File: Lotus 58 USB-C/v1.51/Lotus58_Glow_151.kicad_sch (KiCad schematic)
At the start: 151 parts, among them J1 HRO-TYPE-C-31-M-13x, P1 OLED, SW1 Kailh hotswap MX socket, SW10 Kailh hotswap MX socket, SW11 Kailh hotswap MX socket, SW12 Kailh hotswap MX socket, SW13 Kailh hotswap MX socket, SW14 Kailh hotswap MX socket, SW15 Kailh hotswap MX socket, SW16 Kailh hotswap MX socket, SW17 Kailh hotswap MX socket, SW18 Kailh hotswap MX socket, SW19 Kailh hotswap MX socket, SW2 Kailh hotswap MX socket, SW20 Kailh hotswap MX socket, SW21 Kailh hotswap MX socket, SW22 Kailh hotswap MX socket, SW23 Kailh hotswap MX socket, SW24 Kailh hotswap MX socket, SW25 Kailh hotswap MX socket, SW26 Kailh hotswap MX socket, SW27 Kailh hotswap MX socket, SW28 Kailh hotswap MX socket, SW29 Kailh hotswap MX socket, SW3 Kailh hotswap MX socket, SW4 Kailh hotswap MX socket, SW5 Kailh hotswap MX socket, SW6 Kailh hotswap MX socket, SW7 Kailh hotswap MX socket, SW8 Kailh hotswap MX socket, SW9 Kailh hotswap MX socket, U1 Controller, U2 SRV05-4, U3 SRV05-4

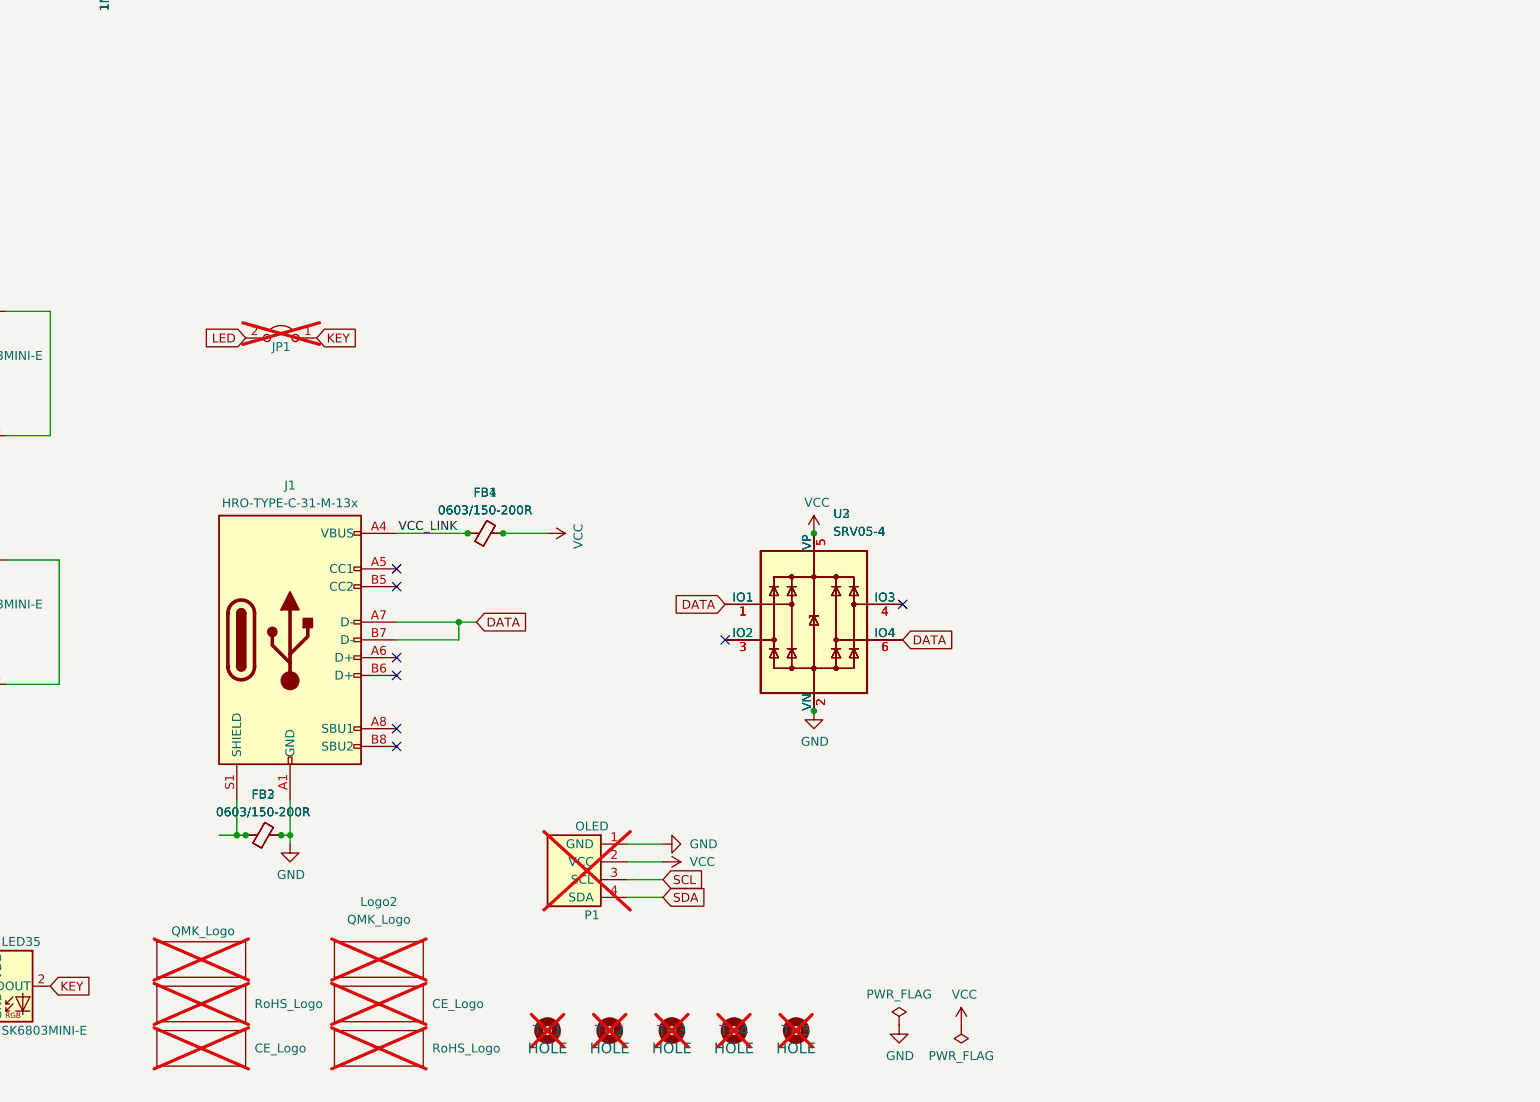
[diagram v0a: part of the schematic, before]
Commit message: Lotus 58 - TRRS Link v1.30
release ready

Signed-off-by: Markus Knutsson <markus.knutsson@tweety.se>
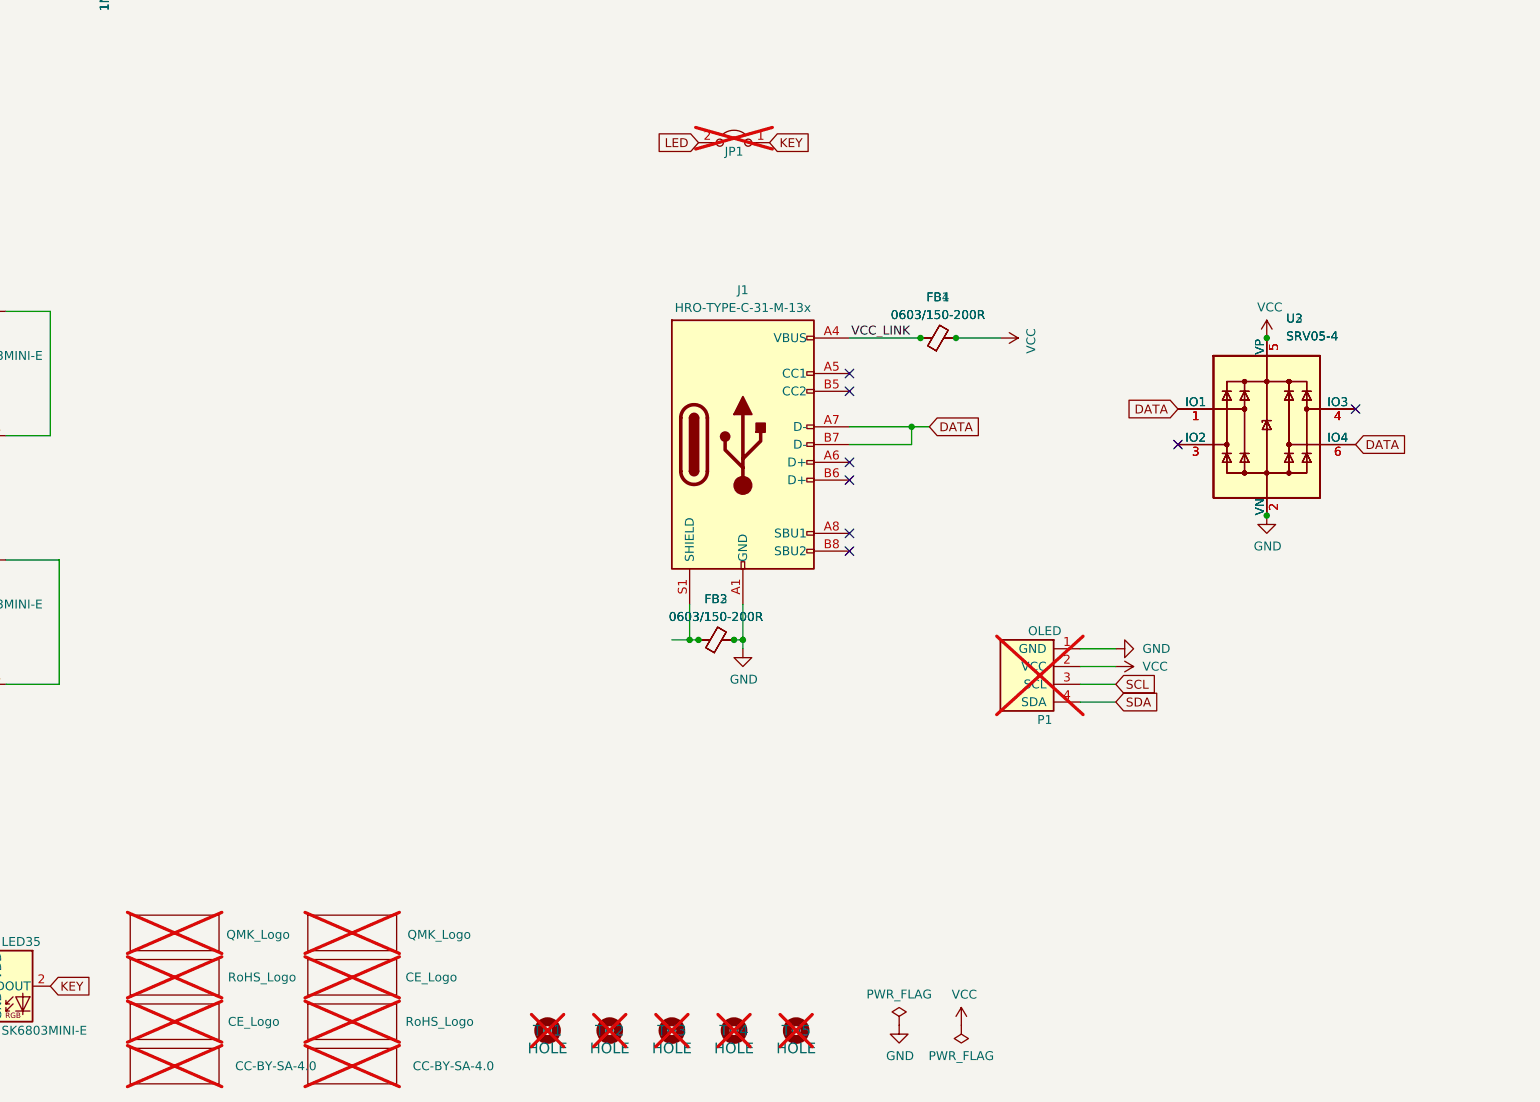
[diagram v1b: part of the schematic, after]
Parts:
- added Logo7, Logo8: CC-BY-SA-4.0, Logotypes:CC_BY_SA_40_line, symbol Logotypes:CC-BY-SA-4.0
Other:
- moved on the sheet: FB1, FB2, FB3, FB4, J1, JP1, P1, U2, U3
